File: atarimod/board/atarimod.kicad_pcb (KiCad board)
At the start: 2 copper layers, 24.1 x 50.8 mm, 15 parts, among them IC1 74HC14D, IC2 74HC14D, IC3 74HC14D, IC4 74HC14D, P1 CONN_02X20, P2 CONN_02X10, U2 APE8865N-33-HF-3

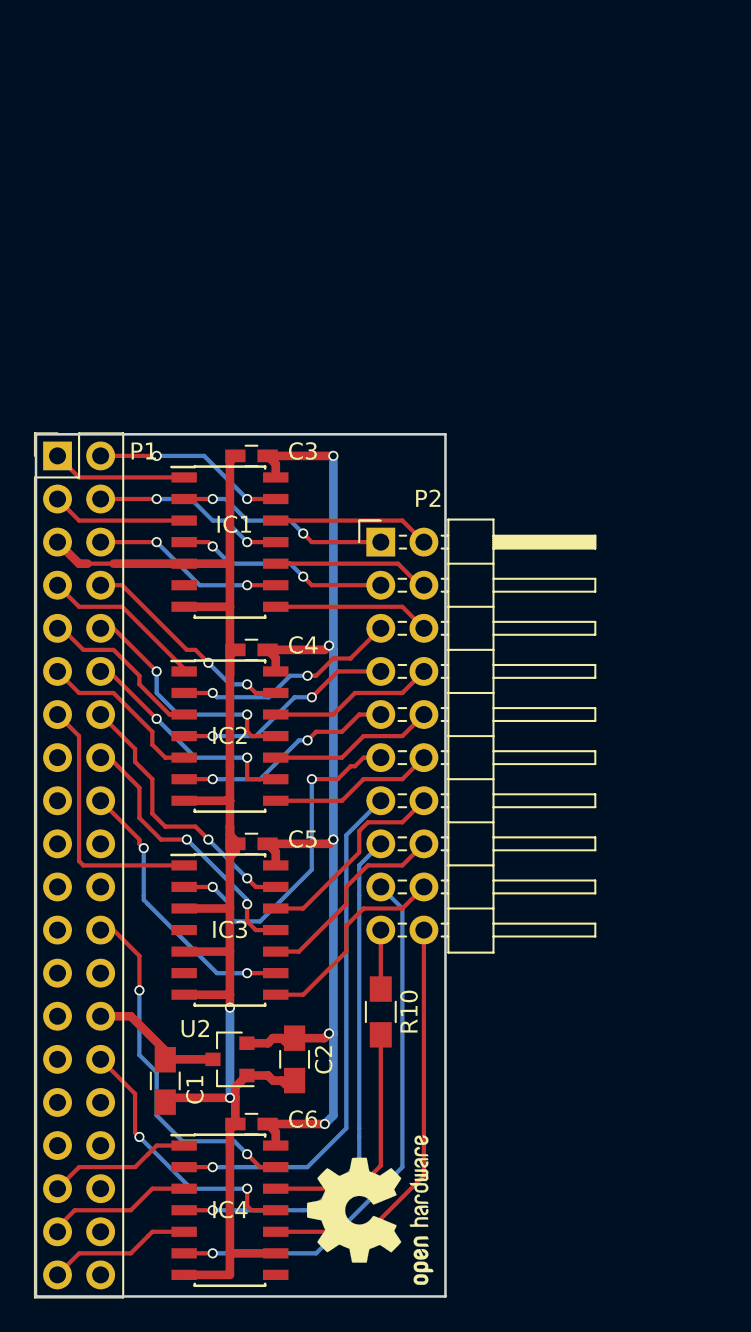
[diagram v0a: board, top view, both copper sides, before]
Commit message: Revision 3 of Atari GTIA Adapter
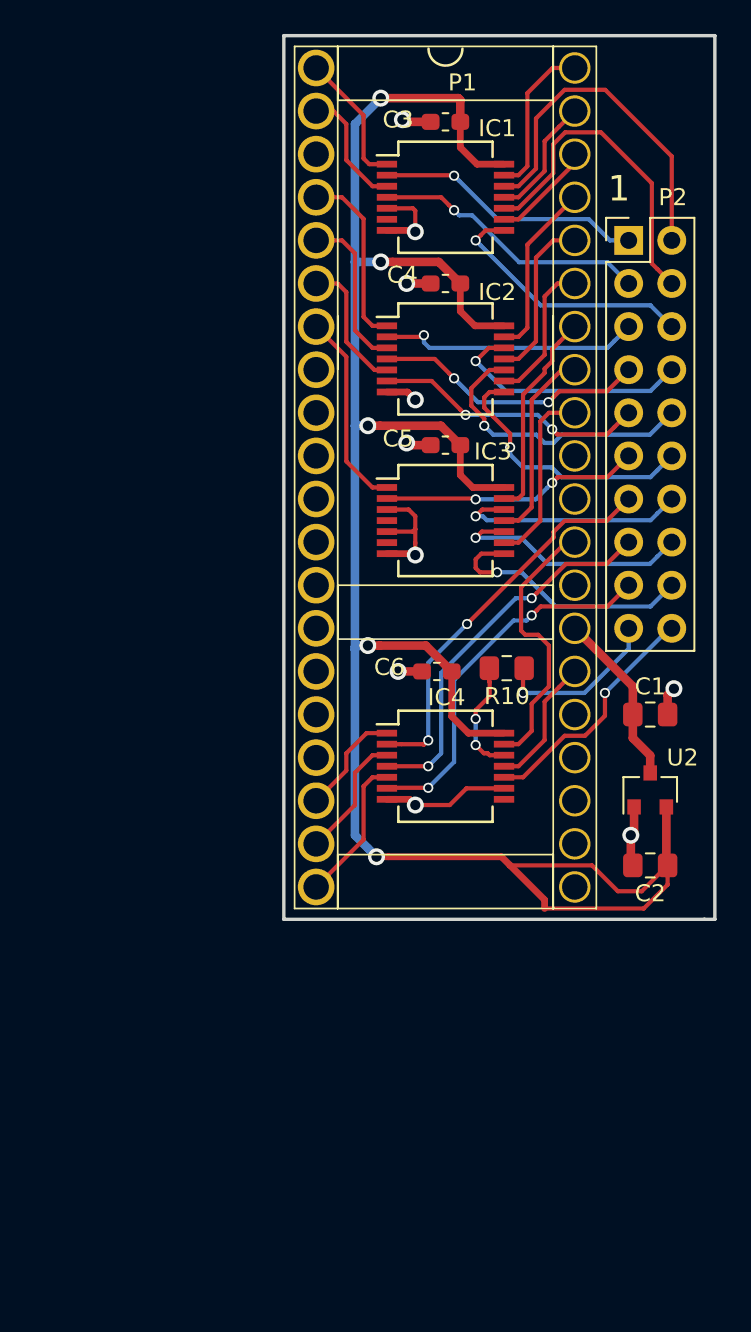
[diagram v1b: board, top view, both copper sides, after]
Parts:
- removed REF***: OSHW-Logo2_9.8x8mm_SilkScreen, Symbols:OSHW-Logo2_9.8x8mm_SilkScreen
- C1, C2: value 10uF -> 1uF; footprint Capacitors_SMD:C_0805_HandSoldering -> Capacitor_SMD:C_0805_2012Metric_Pad1.15x1.40mm_HandSolder
- C3, C4, C5, C6: footprint Capacitors_SMD:C_0603_HandSoldering -> Capacitor_SMD:C_0603_1608Metric_Pad1.05x0.95mm_HandSolder
- IC1, IC2, IC3, IC4: value 74HC14D -> SN74LVC14ADBR; footprint Housings_SOIC:SOIC-14_3.9x8.7mm_Pitch1.27mm -> Package_SO:SSOP-14_5.3x6.2mm_P0.65mm
- P1: value CONN_02X20 -> DIP40_Socket; footprint Pin_Headers:Pin_Header_Straight_2x20_Pitch2.54mm -> ProjectFootprints:socket_embedded_40pin
- P2: footprint Pin_Headers:Pin_Header_Angled_2x10_Pitch2.54mm -> Connector_PinHeader_2.54mm:PinHeader_2x10_P2.54mm_Vertical
- R10: footprint Resistors_SMD:R_0805_HandSoldering -> Resistor_SMD:R_0805_2012Metric_Pad1.15x1.40mm_HandSolder
- U2: value APE8865N-33-HF-3 -> RT9166-33GVL; footprint TO_SOT_Packages_SMD:SOT-23 -> Package_TO_SOT_SMD:SOT-23
- moved C1 35.8 mm to (144.1, 99.1), turned to 0 degrees
- moved U2 29.4 mm to (144.1, 103.5), turned to 90 degrees
- moved IC4 29.1 mm to (132.1, 102.1)
- moved C6 28.8 mm to (131.6, 96.5)
- moved IC3 27.3 mm to (132.1, 87.6)
- moved C5 26.1 mm to (132.1, 83.2)
- moved IC2 25.6 mm to (132.1, 78.1)
- moved C4 24.4 mm to (132.1, 73.7)
- moved IC1 24.0 mm to (132.1, 68.6)
- moved C2 23.9 mm to (144.1, 108.0), turned to 180 degrees
- moved P2 23.0 mm to (142.9, 71.1)
- moved P1 22.9 mm to (132.1, 83.8), turned to 270 degrees
- moved C3 22.8 mm to (132.1, 64.1)
- moved R10 21.6 mm to (135.7, 96.3), turned to 180 degrees
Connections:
- IC1 pad 6: (no net) -> Net-(IC1-Pad6)
- IC3 pad 4: (no net) -> Net-(IC3-Pad4)
- IC3 pad 6: (no net) -> Net-(IC3-Pad6)
- IC4 pad 8: (no net) -> Net-(IC4-Pad8)
- P1 pad 10: Net-(IC2-Pad11) -> Net-(P1-Pad10)
- P1 pad 11: Net-(IC2-Pad5) -> Net-(P1-Pad11)
- P1 pad 12: Net-(IC2-Pad9) -> Net-(P1-Pad12)
- P1 pad 13: Net-(IC3-Pad1) -> Net-(P1-Pad13)
- P1 pad 14: Net-(IC3-Pad13) -> Net-(P1-Pad14)
- P1 pad 15: (no net) -> Net-(P1-Pad15)
- P1 pad 16: Net-(IC3-Pad11) -> Net-(P1-Pad16)
- P1 pad 17: (no net) -> Net-(P1-Pad17)
- P1 pad 18: Net-(IC3-Pad9) -> Net-(IC4-Pad1)
- P1 pad 19: (no net) -> Net-(IC4-Pad3)
- P1 pad 2: Net-(IC1-Pad13) -> Net-(IC1-Pad3)
- P1 pad 20: (no net) -> Net-(IC4-Pad5)
- P1 pad 21: (no net) -> Net-(P1-Pad21)
- P1 pad 22: (no net) -> Net-(P1-Pad22)
- P1 pad 23: (no net) -> Net-(P1-Pad23)
- P1 pad 24: Net-(IC4-Pad13) -> Net-(P1-Pad24)
- P1 pad 25: (no net) -> Net-(P1-Pad25)
- P1 pad 26: (no net) -> Net-(IC4-Pad11)
- P1 pad 27: (no net) -> +5V
- P1 pad 28: +5V -> Net-(P1-Pad28)
- P1 pad 29: (no net) -> Net-(IC4-Pad13)
- P1 pad 3: Net-(IC1-Pad3) -> GND
- P1 pad 30: Net-(IC4-Pad11) -> Net-(P1-Pad30)
- P1 pad 31: (no net) -> Net-(P1-Pad31)
- P1 pad 32: (no net) -> Net-(IC3-Pad9)
- P1 pad 33: (no net) -> Net-(IC3-Pad11)
- P1 pad 34: (no net) -> Net-(IC3-Pad13)
- P1 pad 35: Net-(IC4-Pad1) -> Net-(IC2-Pad9)
- P1 pad 36: (no net) -> Net-(IC2-Pad11)
- P1 pad 37: Net-(IC4-Pad3) -> Net-(IC2-Pad13)
- P1 pad 38: (no net) -> Net-(IC1-Pad9)
- P1 pad 39: Net-(IC4-Pad5) -> Net-(IC1-Pad11)
- P1 pad 4: Net-(IC1-Pad11) -> Net-(IC2-Pad1)
- P1 pad 40: (no net) -> Net-(IC1-Pad13)
- P1 pad 5: GND -> Net-(IC2-Pad3)
- P1 pad 6: Net-(IC1-Pad9) -> Net-(IC2-Pad5)
- P1 pad 7: Net-(IC2-Pad1) -> Net-(IC3-Pad1)
- P1 pad 8: Net-(IC2-Pad13) -> Net-(P1-Pad8)
- P1 pad 9: Net-(IC2-Pad3) -> Net-(P1-Pad9)
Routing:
- net +3V3: track 67.2 -> 126.2 mm
- net GND: track 91.0 -> 32.8 mm, vias 2 -> 10
- net A2: track 9.26 -> 20.6 mm
- net HALT: track 24.6 -> 14.3 mm, vias 0 -> 1
- net AN2: track 32.0 -> 22.0 mm, vias 1 -> 2
- net A3: track 9.26 -> 19.2 mm
- net AN1: track 30.8 -> 22.5 mm, vias 1 -> 2
- net Net-(IC4-Pad11): track 15.9 -> 7.81 mm, vias 2 -> 0
- net CLK: track 14.5 -> 6.80 mm, vias 0 -> 2
- net AN0: track 30.7 -> 23.1 mm, vias 1 -> 2
- net D5: track 9.78 -> 17.1 mm, vias 0 -> 1
- net Net-(P2-Pad19): track 3.48 -> 9.99 mm, vias 0 -> 1
- net A4: track 9.26 -> 15.6 mm, vias 0 -> 1
- net D6: track 9.78 -> 15.9 mm, vias 0 -> 1
- net Net-(IC3-Pad9): track 16.5 -> 10.8 mm, vias 2 -> 0
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- added copper zone on B.Cu, net GND
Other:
- board size 24.1 x 50.8 mm -> 25.4 x 52.1 mm
- board text added: "1"
- board text added: "Atari GTIA Adapter Rev. 3 github.com/c0pperdragon/A-VideoBoard"
